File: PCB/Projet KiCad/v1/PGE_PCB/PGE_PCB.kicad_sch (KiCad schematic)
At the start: 50 parts, among them CN2 Conn_01x02, J1 Conn_01x03, P1 USB_C_Plug_USB2.0, SW1 SW_Push, U1 STM32L476RGTx, U2 MCP73831T, U3 DS2438AZ+, U4 LD39050PU33R, U5 SiP32431DR3, Y1 ABS25-32.768KHZ-T

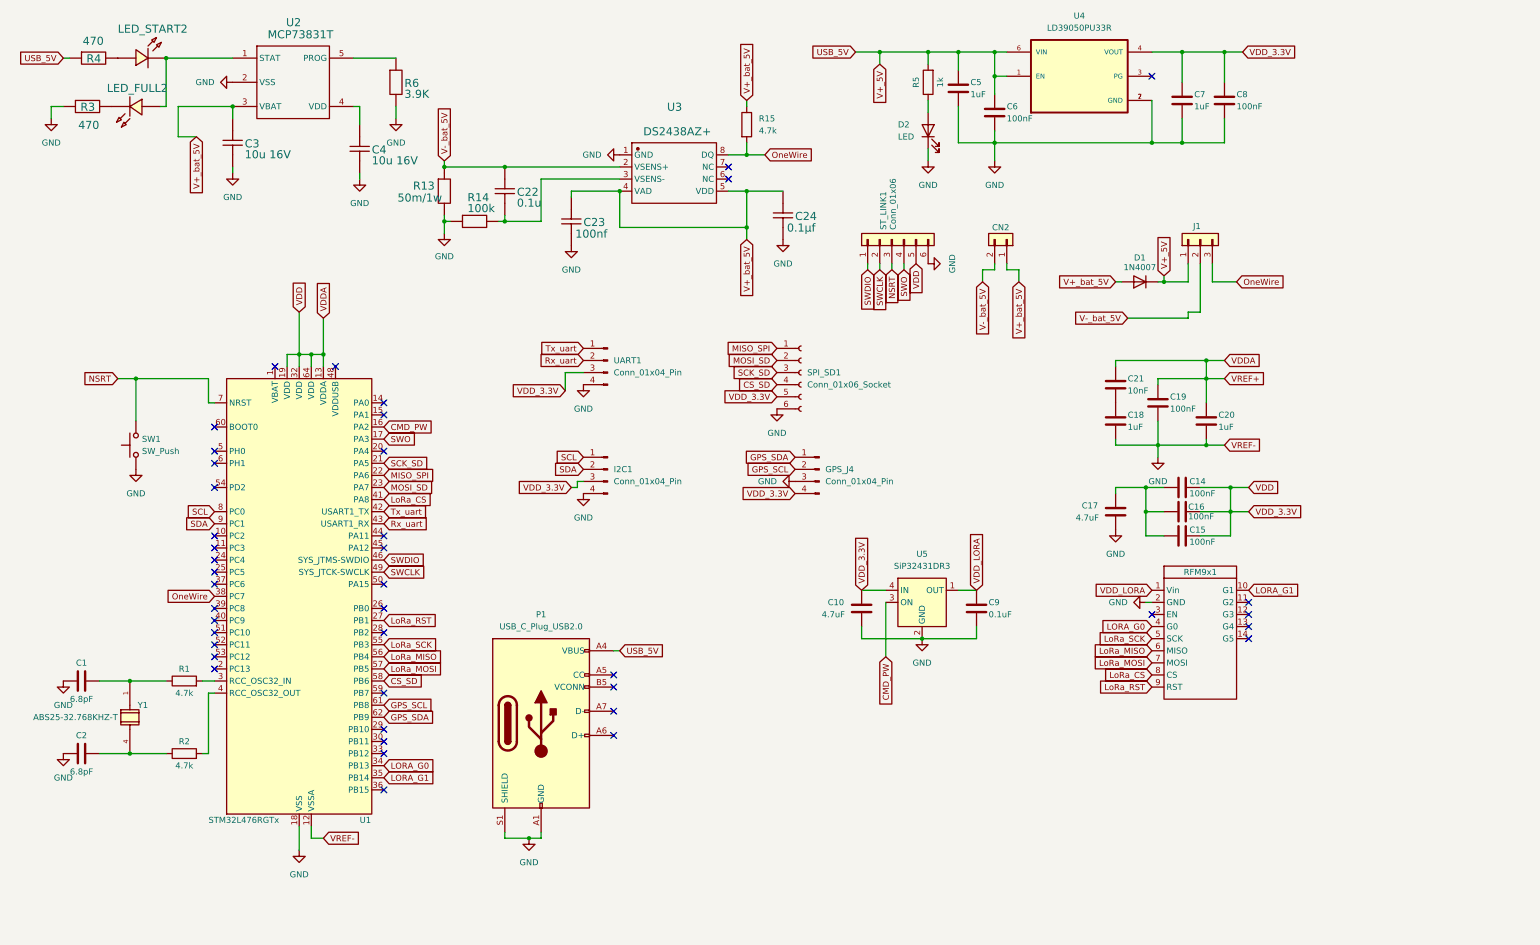
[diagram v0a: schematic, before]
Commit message: Pcb VERSION GPS séparer
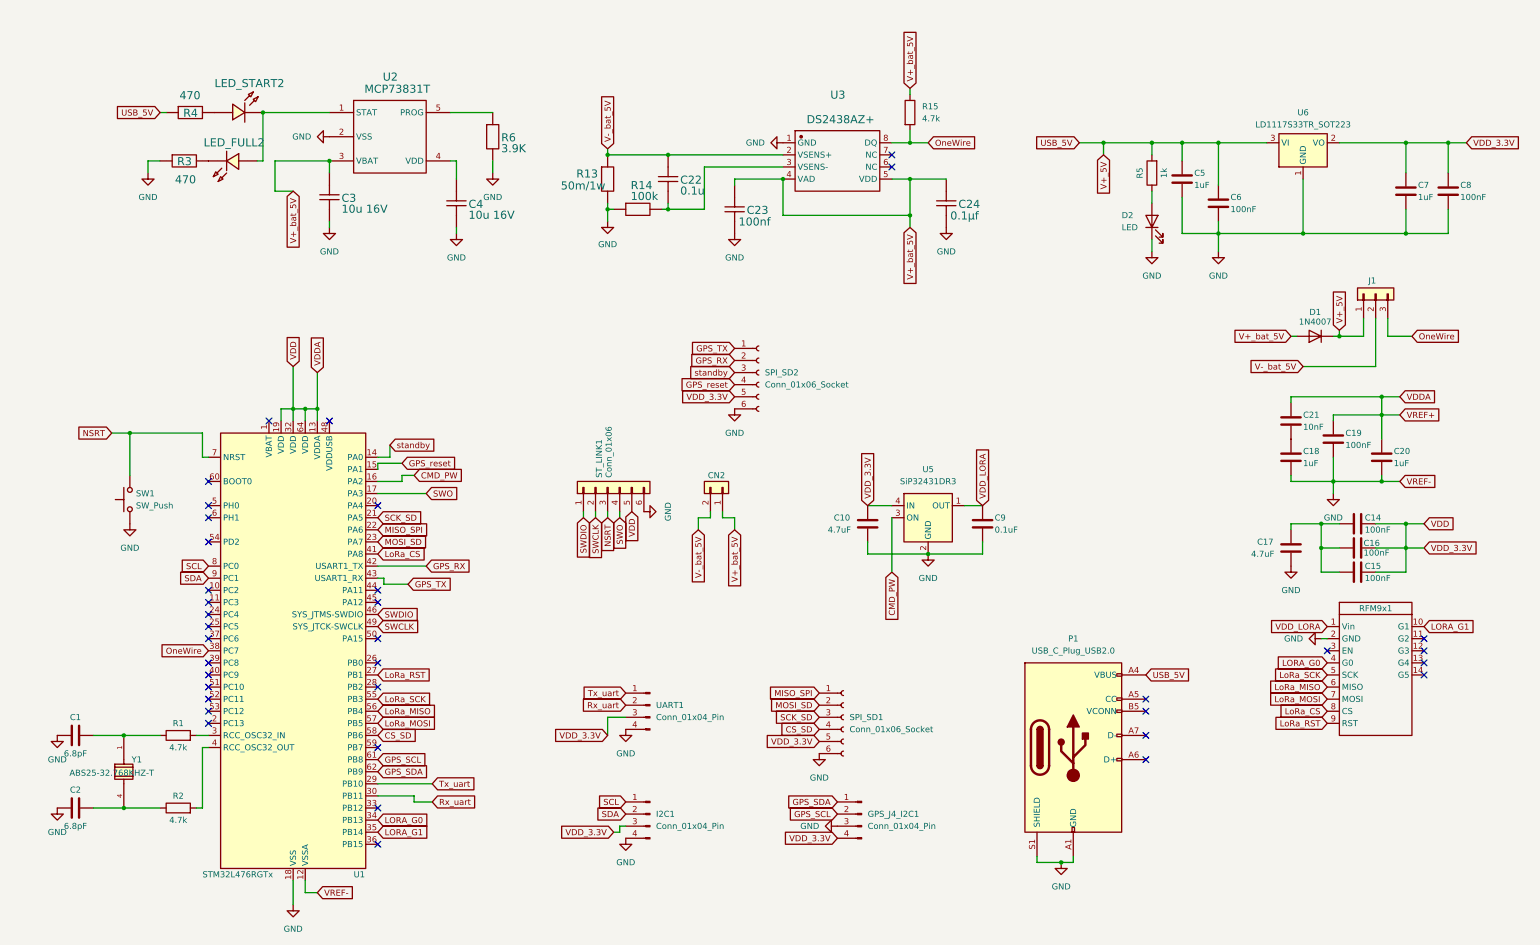
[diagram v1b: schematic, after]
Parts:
- removed U4: LD39050PU33R, Package_DFN_QFN:DFN-6-1EP_3x3mm_P0.95mm_EP1.7x2.6mm, symbol LD39050PU33R:LD39050PU33R
- added SPI_SD2: Conn_01x06_Socket, Connector_PinHeader_2.54mm:PinHeader_1x06_P2.54mm_Vertical, symbol Connector:Conn_01x06_Socket
- added U6: LD1117S33TR_SOT223, Package_TO_SOT_SMD:SOT-223-3_TabPin2, symbol Regulator_Linear:LD1117S33TR_SOT223
- P1: footprint Connector_USB:USB_C_Plug_Molex_105444 -> Connector_USB:USB_C_Receptacle_Palconn_UTC16-G
- renumbered GPS_J4 to GPS_J4_I2C1
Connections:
- net GND: now also SPI_SD2.6 (Pin_6), U6.1 (GND)
- net Rx_uart: now also U1.30 (PB11); no longer U1.43 (PA10)
- net Tx_uart: now also U1.29 (PB10); no longer U1.42 (PA9)
- net USB_5V: now also U6.3 (VI)
- net VDD: now also SPI_SD2.5 (Pin_5), U6.2 (VO)
- net standby: now reaches U1.14 (PA0)
- net standby: now also SPI_SD2.3 (Pin_3)
- net GPS_reset: now reaches U1.15 (PA1)
- net GPS_reset: now also SPI_SD2.4 (Pin_4)
- new net GPS_RX: SPI_SD2.2 (Pin_2), U1.42 (PA9)
- new net GPS_TX: SPI_SD2.1 (Pin_1), U1.43 (PA10)
- no-connect marks 42 -> 37
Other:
- moved on the sheet: C1, C10, C14, C15, C16, C17, C18, C19, C2, C20, C21, C22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
